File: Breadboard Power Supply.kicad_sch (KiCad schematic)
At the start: 29 parts, among them J1 USB-C, J10 Conn_01x02_Male, J11 Conn_01x02_Male, J2 Conn_02x03_Odd_Even, J3 Conn_02x03_Odd_Even, J8 Conn_01x02_Male, J9 Conn_01x02_Male, U1 LM1117-1.8, U2 LM1117-3.3

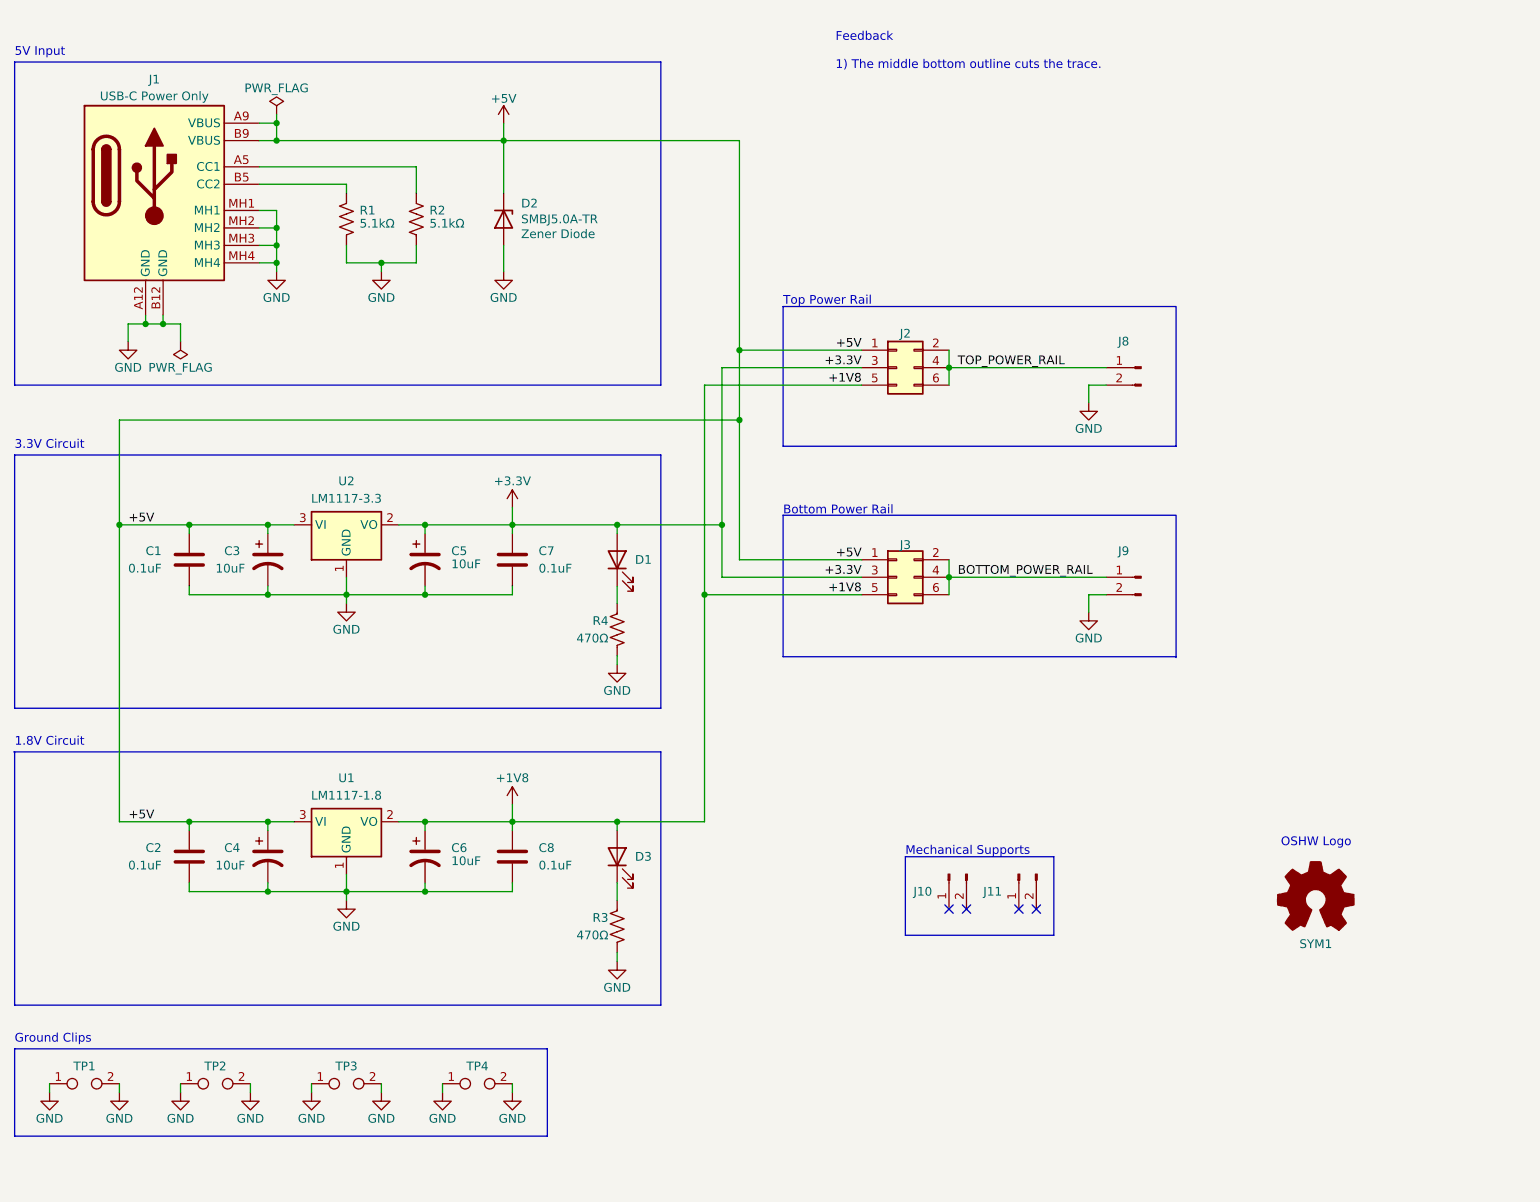
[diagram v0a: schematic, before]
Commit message: Added feedback.
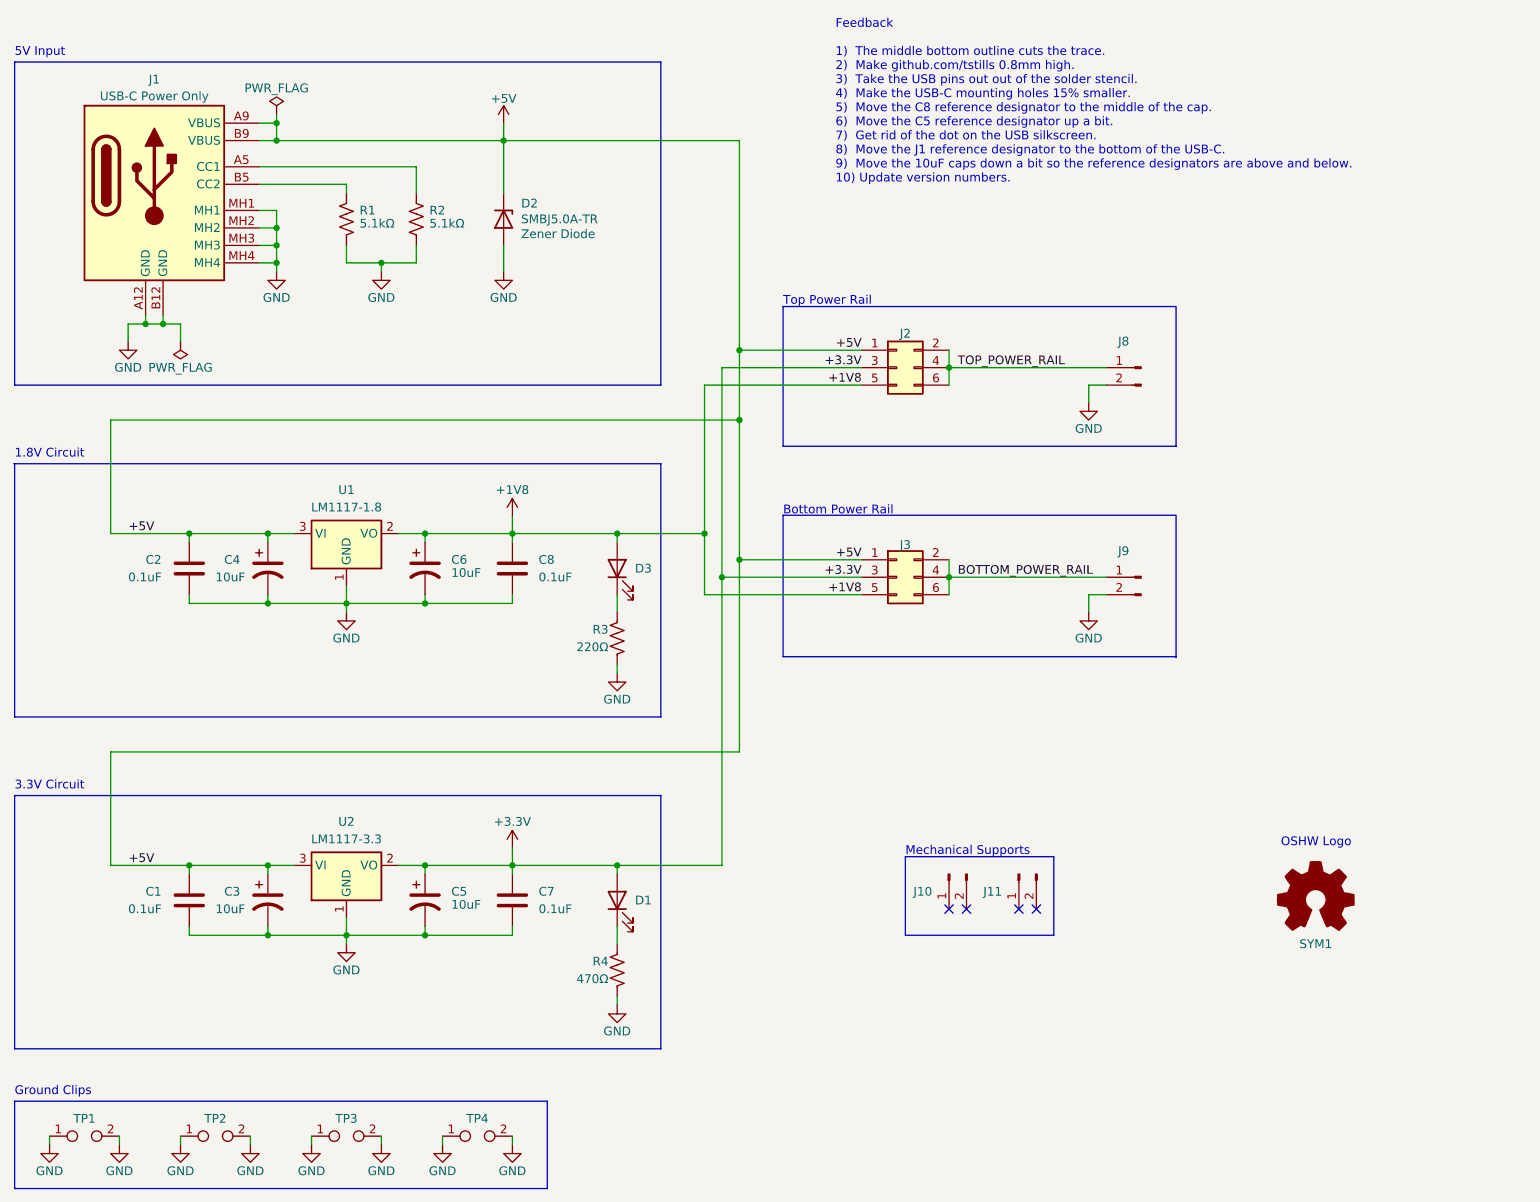
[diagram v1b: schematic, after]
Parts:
- R3: value 470Ω -> 220Ω
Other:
- note added: "Feedback 1) The middle bottom outline cuts the trace. 2) Make github.com/tstills 0.8mm high. 3) Take the USB pins out out of the solder stencil. 4) Make the USB-C mounting holes 15% smaller. 5) Move the C8 reference designator to the middle of the cap. 6) Move the C5 reference designator up a bit. 7) Get rid of the dot on the USB silkscreen. 8) Move the J1 reference designator to the bottom of th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"
- note removed: "Feedback 1) The middle bottom outline cuts the trace."
- moved on the sheet: C1, C2, C3, C4, C5, C6, C7, C8, D1, D3, R3, R4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
